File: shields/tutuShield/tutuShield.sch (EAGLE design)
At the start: 23 parts, among them IC1 IC_MSGEQ7-SOIC8, Q4 2N3904

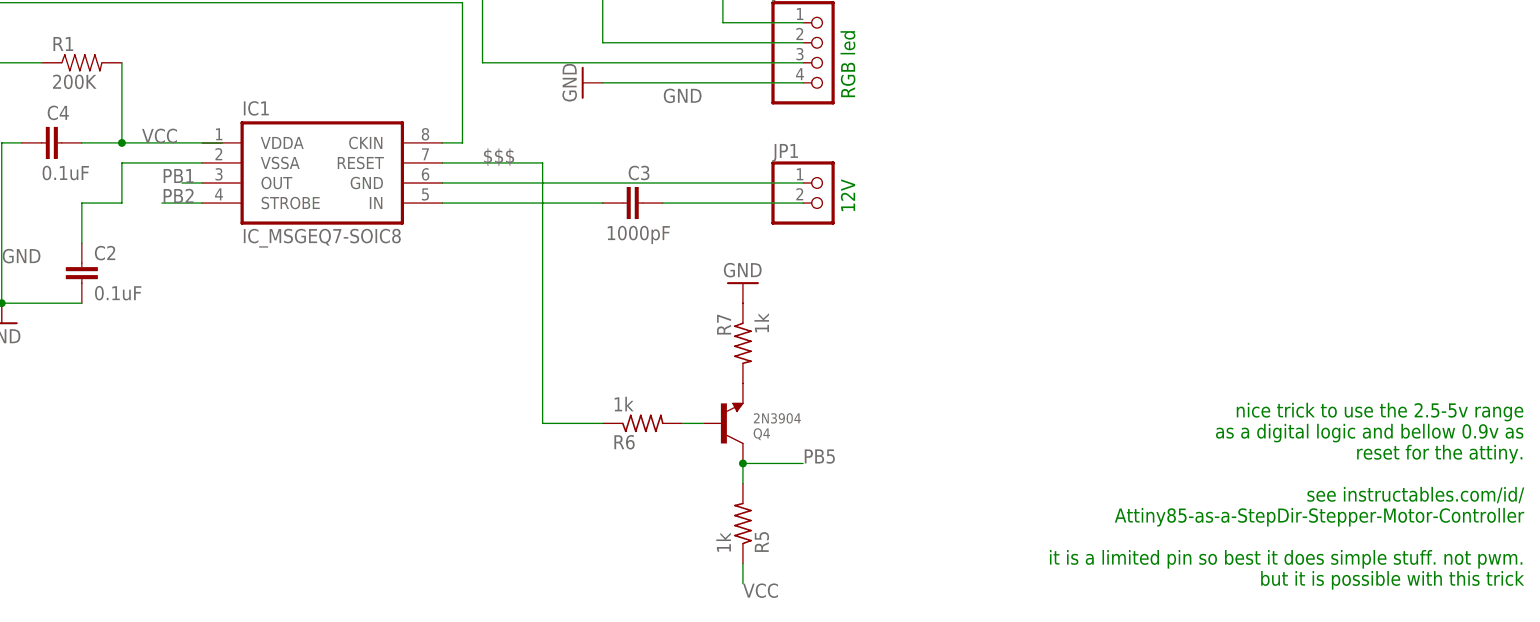
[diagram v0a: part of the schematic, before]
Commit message: sorry, i mixed signals
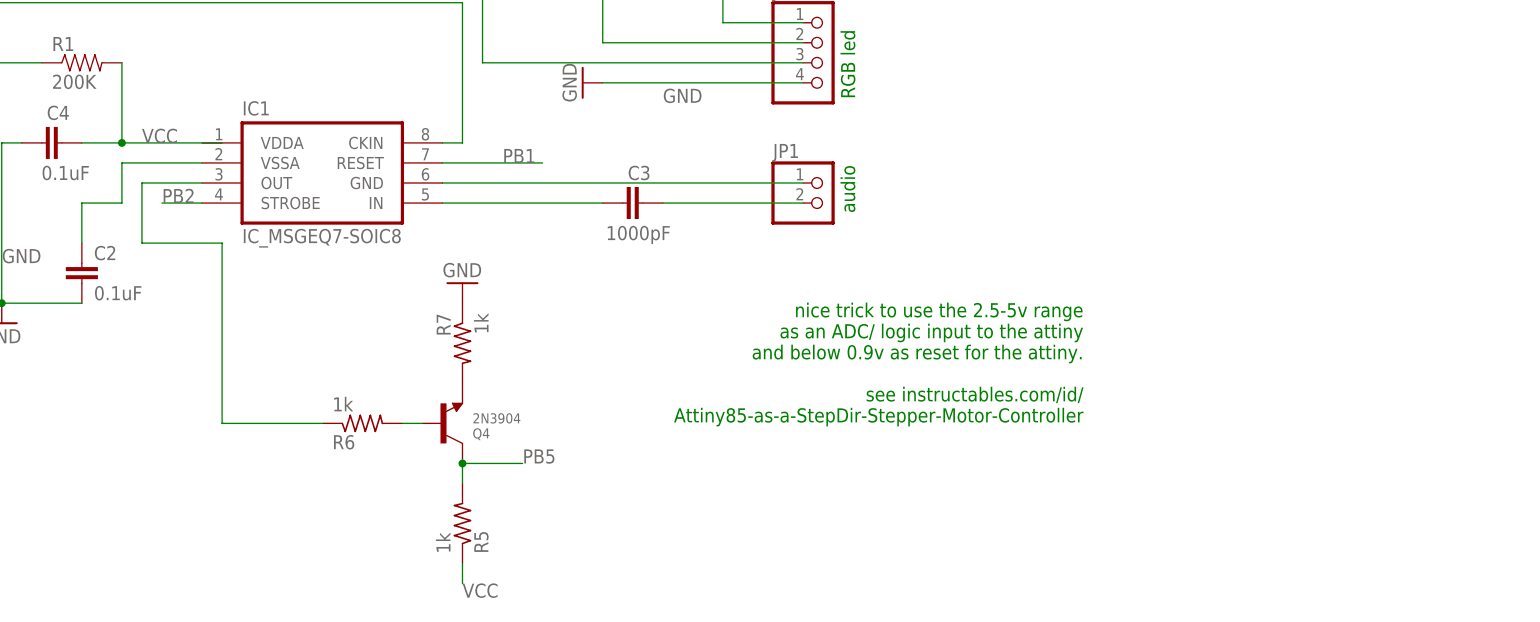
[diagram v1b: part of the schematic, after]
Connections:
- removed net $$$: IC1.RESET, R6.1
- net PB1: now also IC1.RESET, R6.1
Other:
- note added: "audio"
- note added: "nice trick to use the 2.5-5v range as an ADC/ logic input to the attiny and below 0.9v as reset for the attiny. see instructables.com/id/ Attiny85-as-a-StepDir-Stepper-Motor-Controller"
- note removed: "12V"
- note removed: "nice trick to use the 2.5-5v range as a digital logic and bellow 0.9v as reset for the attiny. see instructables.com/id/ Attiny85-as-a-StepDir-Stepper-Motor-Controller it is a limited pin so best it does simple stuff. not pwm. but it is possible with this trick"
- moved on the sheet: Q4, R5, R6, R7
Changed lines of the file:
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@@
 as a digital logic and bellow 0.9v as reset.
 see instructables.com/id/Attiny85-as-a-StepDir-Stepper-Motor-Controller</text>
-<text x="269.24" y="55.88" size="1.778" layer="91" rot="R180">nice trick to use the 2.5-5v range
-as a digital logic and bellow 0.9v as
-reset for the attiny.
+<text x="213.36" y="68.58" size="1.778" layer="91" rot="R180">nice trick to use the 2.5-5v range
+as an ADC/ logic input to the attiny
+and below 0.9v as reset for the attiny.
 see instructables.com/id/
 Attiny85-as-a-StepDir-Stepper-Motor-Controller
-it is a limited pin so best it does simple stuff. not pwm.
-but it is possible with this trick</text>
-<text x="184.404" y="80.01" size="1.778" layer="91" rot="R90">12V</text>
+</text>
+<text x="184.404" y="80.01" size="1.778" layer="91" rot="R90">audio</text>
 <text x="184.404" y="94.488" size="1.778" layer="91" rot="R90">RGB led </text>
 </plain>
@@
 <instance part="JP2" gate="A" x="180.34" y="104.14"/>
 <instance part="GND3" gate="1" x="149.86" y="96.52" rot="R270"/>
-<instance part="R5" gate="G$1" x="170.18" y="40.64" rot="MR90"/>
-<instance part="Q4" gate="G$1" x="170.18" y="53.34" rot="MR180"/>
-<instance part="R6" gate="G$1" x="157.48" y="53.34" rot="MR180"/>
-<instance part="R7" gate="G$1" x="170.18" y="63.5" rot="MR270"/>
-<instance part="GND4" gate="1" x="170.18" y="71.12" rot="MR180"/>
+<instance part="R5" gate="G$1" x="134.62" y="40.64" rot="MR90"/>
+<instance part="Q4" gate="G$1" x="134.62" y="53.34" rot="MR180"/>
+<instance part="R6" gate="G$1" x="121.92" y="53.34" rot="MR180"/>
+<instance part="R7" gate="G$1" x="134.62" y="63.5" rot="MR270"/>
+<instance part="GND4" gate="1" x="134.62" y="71.12" rot="MR180"/>
 </instances>
 <busses>
@@
 <segment>
 <pinref part="R5" gate="G$1" pin="1"/>
-<wire x1="170.18" y1="35.56" x2="170.18" y2="33.02" width="0.1524" layer="91"/>
-<label x="170.18" y="33.02" size="1.778" layer="95" rot="MR180"/>
+<wire x1="134.62" y1="35.56" x2="134.62" y2="33.02" width="0.1524" layer="91"/>
+<label x="134.62" y="33.02" size="1.778" layer="95" rot="MR180"/>
 </segment>
 <segment>
@@
 <segment>
 <pinref part="IC1" gate="IC" pin="OUT"/>
-<wire x1="101.6" y1="83.82" x2="99.06" y2="83.82" width="0.1524" layer="91"/>
-<label x="96.52" y="83.82" size="1.778" layer="95"/>
+<wire x1="101.6" y1="83.82" x2="93.98" y2="83.82" width="0.1524" layer="91"/>
+<wire x1="93.98" y1="83.82" x2="93.98" y2="76.2" width="0.1524" layer="91"/>
+<wire x1="93.98" y1="76.2" x2="104.14" y2="76.2" width="0.1524" layer="91"/>
+<wire x1="104.14" y1="76.2" x2="104.14" y2="53.34" width="0.1524" layer="91"/>
+<pinref part="R6" gate="G$1" pin="1"/>
+<wire x1="104.14" y1="53.34" x2="116.84" y2="53.34" width="0.1524" layer="91"/>
+</segment>
+<segment>
+<pinref part="IC1" gate="IC" pin="RESET"/>
+<wire x1="132.08" y1="86.36" x2="144.78" y2="86.36" width="0.1524" layer="91"/>
+<label x="139.7" y="86.36" size="1.778" layer="95"/>
 </segment>
 </net>
@@
 <pinref part="R5" gate="G$1" pin="2"/>
 <pinref part="Q4" gate="G$1" pin="C"/>
-<wire x1="170.18" y1="45.72" x2="170.18" y2="48.26" width="0.1524" layer="91"/>
-<wire x1="170.18" y1="48.26" x2="177.8" y2="48.26" width="0.1524" layer="91"/>
-<junction x="170.18" y="48.26"/>
-<label x="177.8" y="48.26" size="1.778" layer="95"/>
+<wire x1="134.62" y1="45.72" x2="134.62" y2="48.26" width="0.1524" layer="91"/>
+<wire x1="134.62" y1="48.26" x2="142.24" y2="48.26" width="0.1524" layer="91"/>
+<junction x="134.62" y="48.26"/>
+<label x="142.24" y="48.26" size="1.778" layer="95"/>
 </segment>
 </net>
@@
 <pinref part="Q4" gate="G$1" pin="B"/>
 <pinref part="R6" gate="G$1" pin="2"/>
-<wire x1="165.1" y1="53.34" x2="162.56" y2="53.34" width="0.1524" layer="91"/>
-</segment>
-</net>
-<net name="$$$" class="0">
-<segment>
-<pinref part="IC1" gate="IC" pin="RESET"/>
-<wire x1="132.08" y1="86.36" x2="144.78" y2="86.36" width="0.1524" layer="91"/>
-<label x="137.16" y="86.36" size="1.778" layer="95"/>
-<wire x1="144.78" y1="86.36" x2="144.78" y2="53.34" width="0.1524" layer="91"/>
-<pinref part="R6" gate="G$1" pin="1"/>
-<wire x1="144.78" y1="53.34" x2="152.4" y2="53.34" width="0.1524" layer="91"/>
-</segment>
-</net>
+<wire x1="129.54" y1="53.34" x2="127" y2="53.34" width="0.1524" layer="91"/>
+</segment>
+</net>
